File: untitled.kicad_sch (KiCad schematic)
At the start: 62 parts, among them IC5 HX711, IC6 HX711, IC7 HX711, IC8 HX711, J10 Conn_01x04, J15 Conn_01x04, J16 Conn_01x04, J2 Conn_01x04, J6 Conn_01x02, J7 Conn_01x02, Q2 MMBT4403, Q3 MMBT4403, Q4 MMBT4403, Q5 MMBT4403

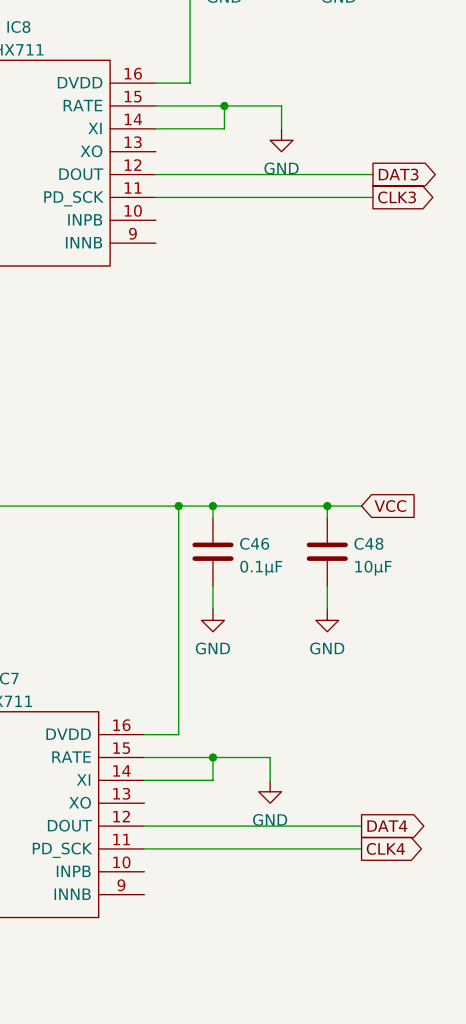
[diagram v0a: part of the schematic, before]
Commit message: update
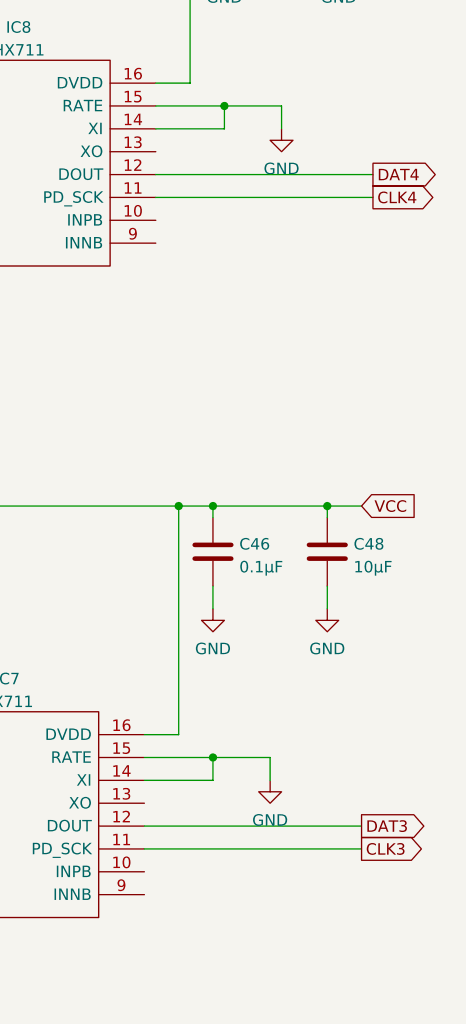
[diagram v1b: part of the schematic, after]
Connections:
- net CLK3: now also IC7.11 (PD_SCK); no longer IC8.11 (PD_SCK)
- net CLK4: now also IC8.11 (PD_SCK); no longer IC7.11 (PD_SCK)
- net DAT3: now also IC7.12 (DOUT); no longer IC8.12 (DOUT)
- net DAT4: now also IC8.12 (DOUT); no longer IC7.12 (DOUT)
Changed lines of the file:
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@@
     (stroke (width 0) (type default) (color 0 0 0 0))
   )
-  (global_label "CLK4" (shape output) (at 276.86 130.81 0) (fields_autoplaced)
+  (global_label "CLK3" (shape output) (at 276.86 130.81 0) (fields_autoplaced)
     (effects (font (size 1.27 1.27)) (justify left))
     (property "Intersheet References" "${INTERSHEET_REFS}" (id 0) (at 283.9618 130.7306 0)
@@
     )
   )
-  (global_label "CLK3" (shape output) (at 278.13 58.42 0) (fields_autoplaced)
+  (global_label "CLK4" (shape output) (at 278.13 58.42 0) (fields_autoplaced)
     (effects (font (size 1.27 1.27)) (justify left))
     (property "Intersheet References" "${INTERSHEET_REFS}" (id 0) (at 285.2318 58.3406 0)
@@
     )
   )
-  (global_label "DAT4" (shape output) (at 276.86 128.27 0) (fields_autoplaced)
+  (global_label "DAT3" (shape output) (at 276.86 128.27 0) (fields_autoplaced)
     (effects (font (size 1.27 1.27)) (justify left))
     (property "Intersheet References" "${INTERSHEET_REFS}" (id 0) (at 283.7199 128.1906 0)
@@
     )
   )
-  (global_label "DAT3" (shape output) (at 278.13 55.88 0) (fields_autoplaced)
+  (global_label "DAT4" (shape output) (at 278.13 55.88 0) (fields_autoplaced)
     (effects (font (size 1.27 1.27)) (justify left))
     (property "Intersheet References" "${INTERSHEET_REFS}" (id 0) (at 284.9899 55.8006 0)
